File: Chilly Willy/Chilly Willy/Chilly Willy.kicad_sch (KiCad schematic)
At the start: 5 parts, among them J2 Screw_Terminal_01x08, J3 Screw_Terminal_01x03, J4 RH+RC

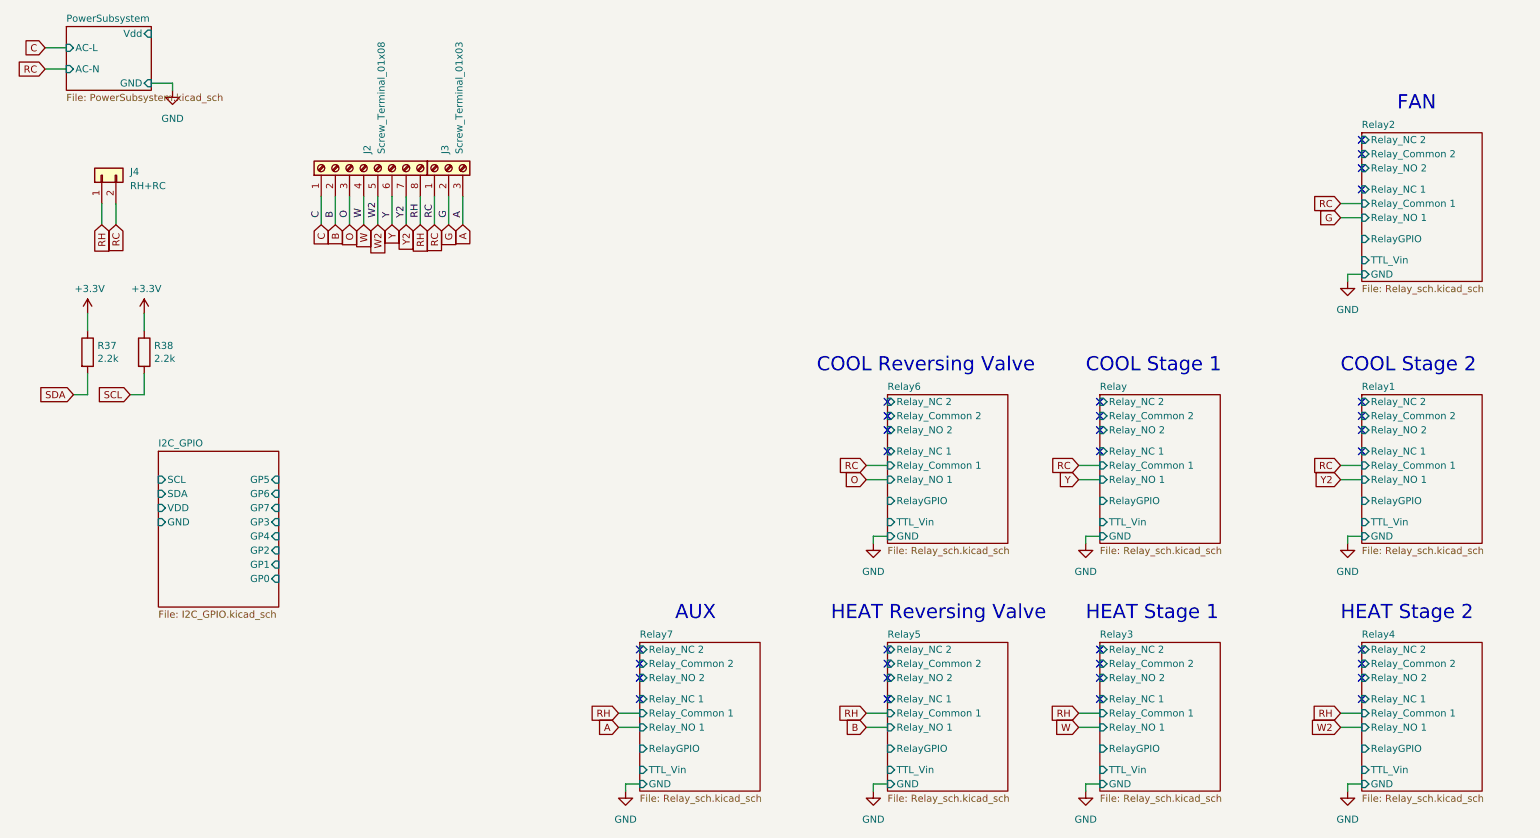
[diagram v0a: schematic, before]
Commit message: ..
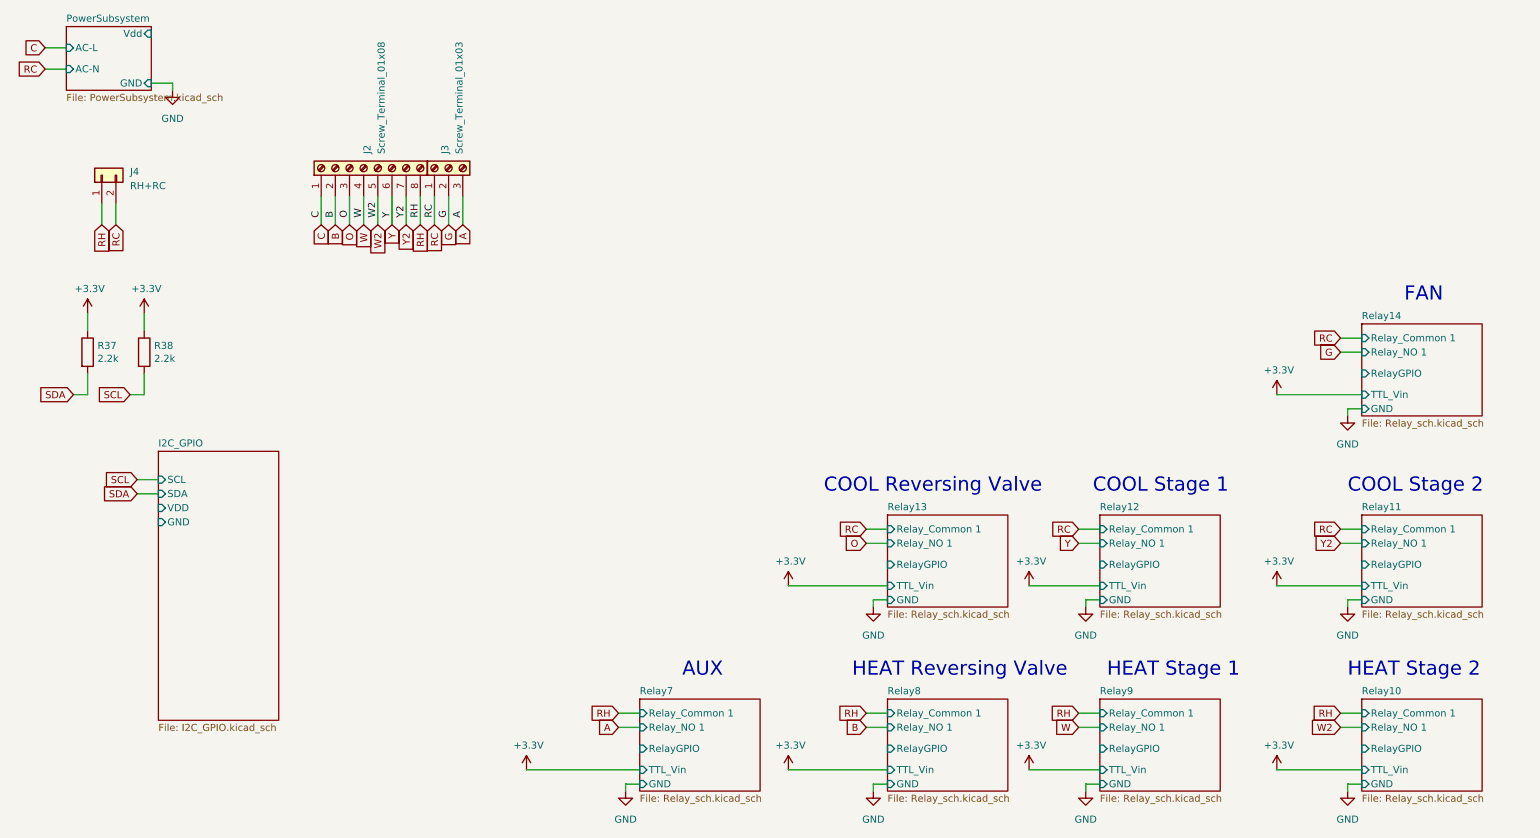
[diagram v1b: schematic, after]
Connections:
- no-connect marks 32 -> 0
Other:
- removed sheet Relay
- removed sheet Relay1
- removed sheet Relay2
- removed sheet Relay3
- removed sheet Relay4
- removed sheet Relay5
- removed sheet Relay6
- added sheet Relay10 (Relay_sch.kicad_sch)
- added sheet Relay11 (Relay_sch.kicad_sch)
- added sheet Relay12 (Relay_sch.kicad_sch)
- added sheet Relay13 (Relay_sch.kicad_sch)
- added sheet Relay14 (Relay_sch.kicad_sch)
- added sheet Relay8 (Relay_sch.kicad_sch)
- added sheet Relay9 (Relay_sch.kicad_sch)
- sheet I2C_GPIO ports: added none; removed GP0, GP1, GP2, GP3, GP4, GP5, GP6, GP7
- sheet Relay7 ports: added none; removed Relay_Common 2 , Relay_NC 1, Relay_NC 2, Relay_NO 2
